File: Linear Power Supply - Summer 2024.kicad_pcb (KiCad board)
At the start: 2 copper layers, 79.5 x 142.5 mm, 4 parts, among them IC1 LD1085V, T1 FP16-3000

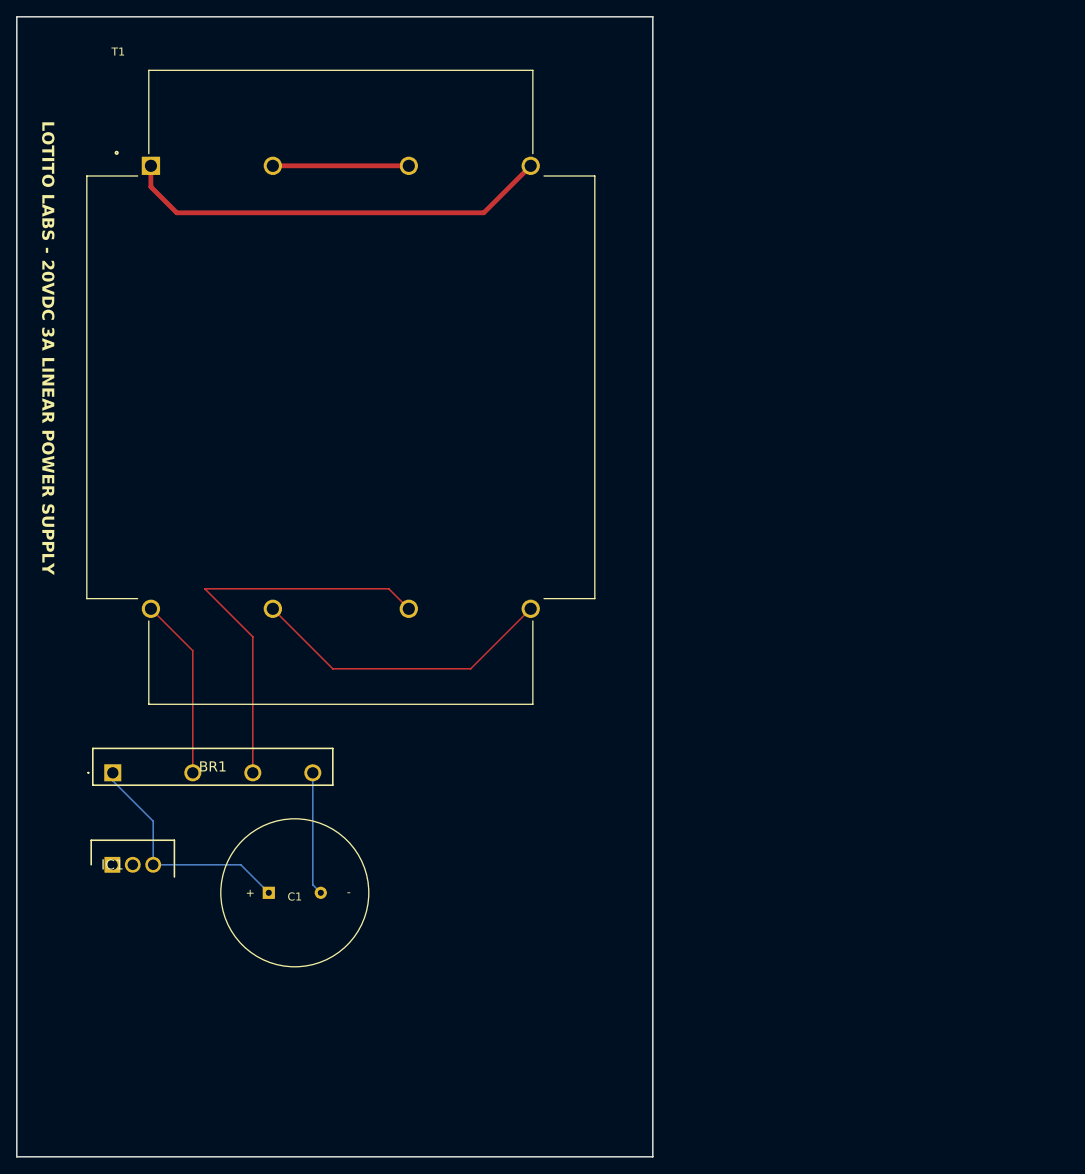
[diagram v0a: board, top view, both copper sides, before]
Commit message: Big push on the PCB layout. I think ready to send to JLC or OSH...
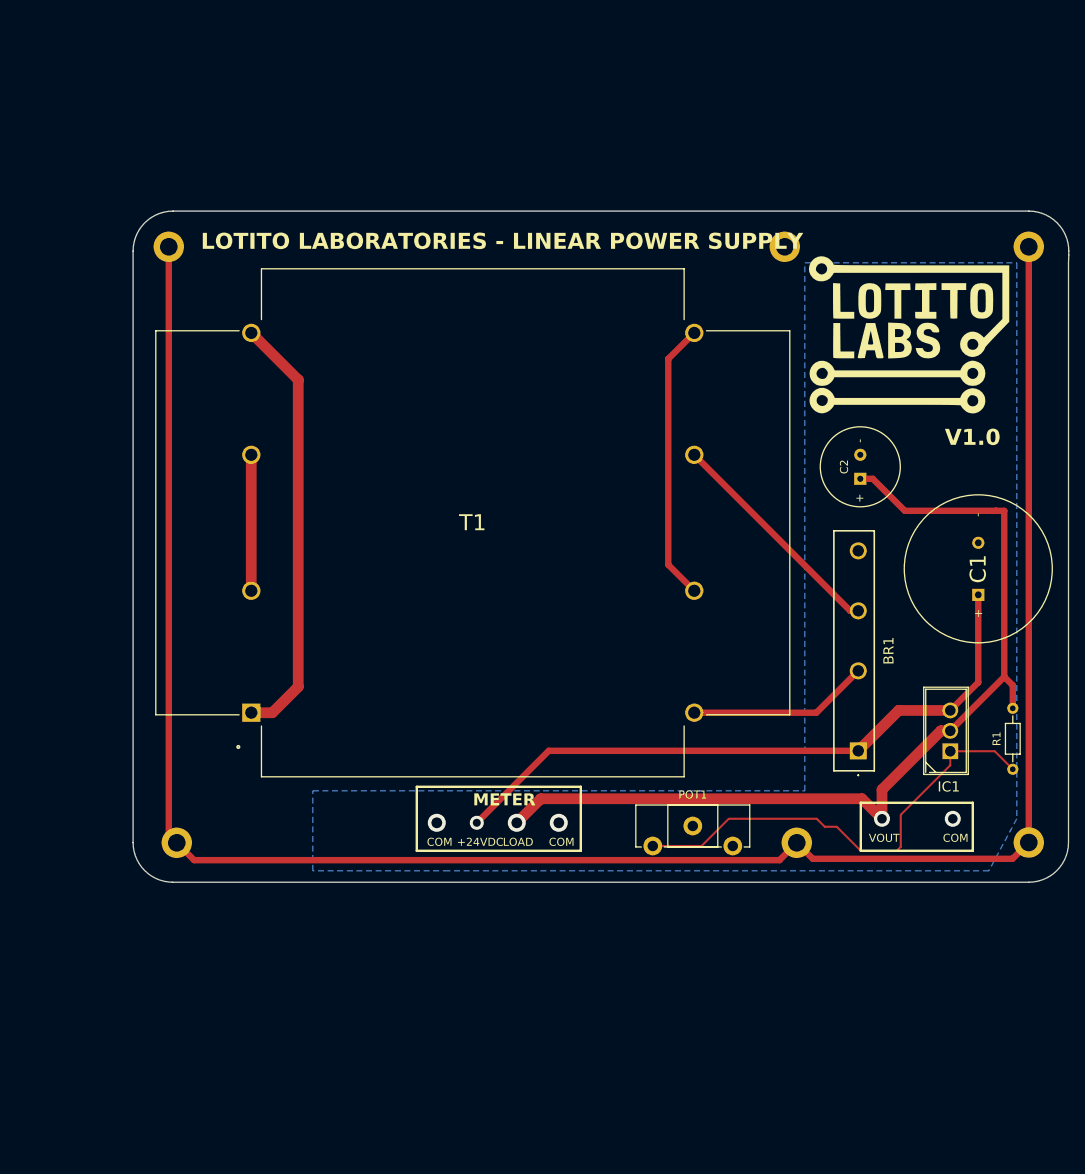
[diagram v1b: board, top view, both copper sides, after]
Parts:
- added C2: 10uF, Chase's Footprints:Small Electrolytic Capacitor, F.Cu at (189.4, 84.5)
- added G***: LOGO, Chase's Footprints:Lotito Labs - 25mm, F.Cu at (195.5, 68.0)
- added POT1: 10k, Potentiometer_THT:Potentiometer_ACP_CA14-H2,5_Horizontal, F.Cu at (163.5, 131.9)
- added R1: 560R, Resistor_THT:R_Axial_DIN0204_L3.6mm_D1.6mm_P7.62mm_Horizontal, F.Cu at (208.5, 114.7)
- added REF**: MountingHole_2.2mm_M2_DIN965_Pad, MountingHole:MountingHole_2.2mm_M2_DIN965_Pad, F.Cu at (104.0, 131.5)
- added REF**: MountingHole_2.2mm_M2_DIN965_Pad, MountingHole:MountingHole_2.2mm_M2_DIN965_Pad, F.Cu at (210.5, 57.0)
- added REF**: MountingHole_2.2mm_M2_DIN965_Pad, MountingHole:MountingHole_2.2mm_M2_DIN965_Pad, F.Cu at (103.0, 57.0)
- added REF**: MountingHole_2.2mm_M2_DIN965_Pad, MountingHole:MountingHole_2.2mm_M2_DIN965_Pad, F.Cu at (181.5, 131.5)
- added REF**: MountingHole_2.2mm_M2_DIN965_Pad, MountingHole:MountingHole_2.2mm_M2_DIN965_Pad, F.Cu at (210.5, 131.5)
- added REF**: MountingHole_2.2mm_M2_DIN965_Pad, MountingHole:MountingHole_2.2mm_M2_DIN965_Pad, F.Cu at (180.0, 57.0)
- moved IC1 105.7 mm to (200.7, 120.1), turned to 90 degrees
- moved C1 94.5 mm to (204.2, 97.3), turned to -90 degrees
- moved BR1 93.2 mm to (189.2, 120.0), turned to 90 degrees
- moved T1 23.6 mm to (141.0, 91.5), turned to 90 degrees
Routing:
- net GND: track 0.00 -> 262.0 mm
- net Vout: track 0.00 -> 117.5 mm, vias 0 -> 2
- net Net-(IC1-ADJ/GND): track 0.00 -> 58.1 mm
- net Net-(BR1-+): track 29.5 -> 81.2 mm, vias 0 -> 1
- net Net-(BR1-~{_2}): track 52.0 -> 28.6 mm
- net COM: track 15.4 -> 0.00 mm, vias 0 -> 3
- net Net-(T1-Pad6): track 38.5 -> 34.9 mm
- added copper zone on B.Cu, net COM
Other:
- board size 79.5 x 142.5 mm -> 117 x 83.9 mm
- board text added: "+24VDC"
- board text added: "COM"
- board text added: "LOAD"
- board text added: "LOTITO LABORATORIES - LINEAR POWER SUPPLY"
- board text added: "METER"
- board text added: "V1.0"
- board text added: "VOUT"
- board text removed: "LOTITO LABS - 20VDC 3A LINEAR POWER SUPPLY"

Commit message: Finished PCB design...
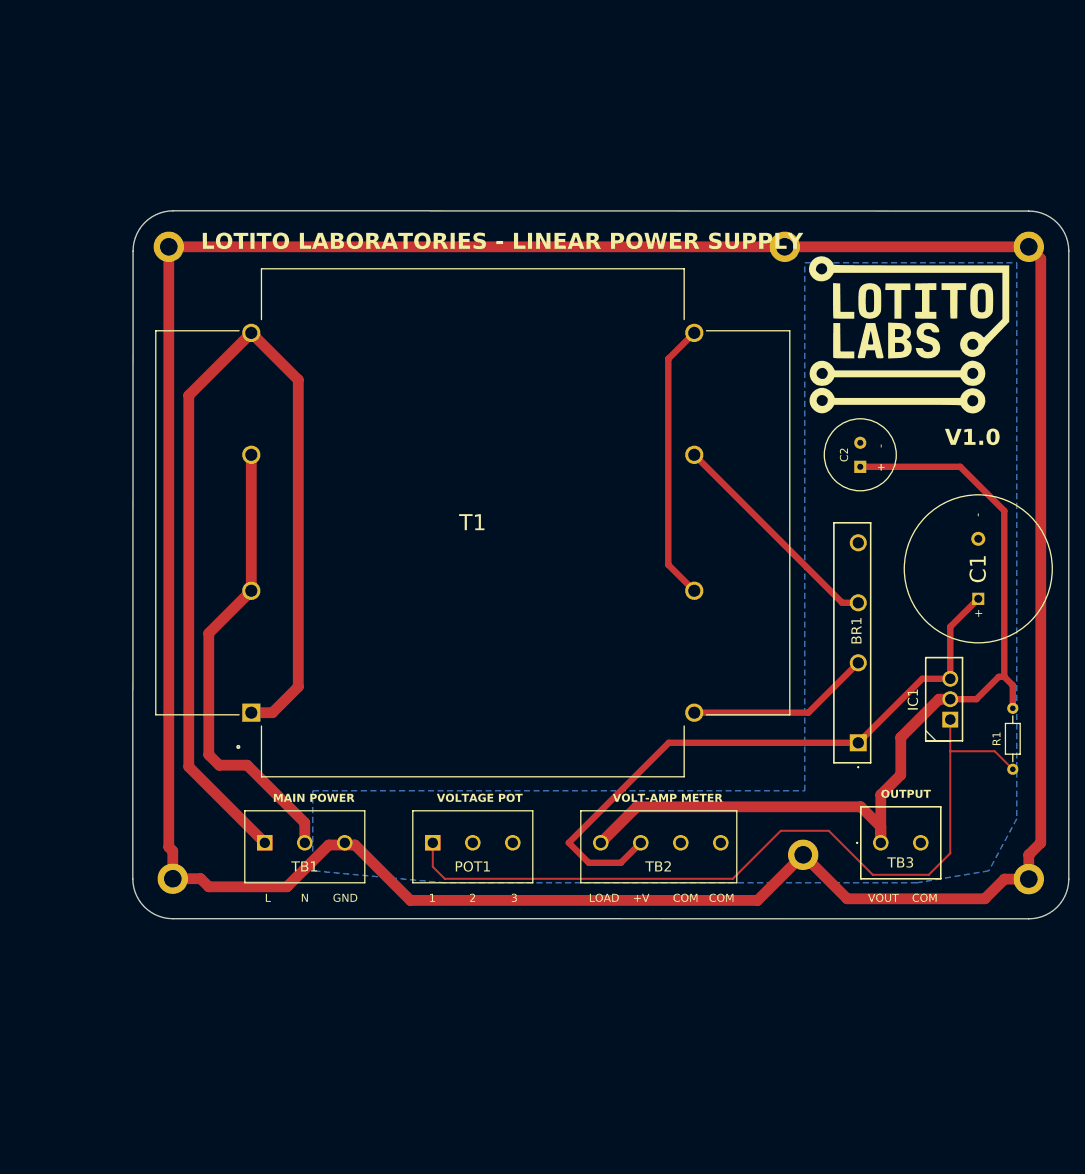
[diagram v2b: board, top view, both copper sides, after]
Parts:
- added TB1: 1935174, SamacSys_PCB_Library:1935174, F.Cu at (115.0, 131.5)
- added TB2: 1935187, SamacSys_PCB_Library:1935187, F.Cu at (157.0, 131.5)
- added TB3: 1935776, SamacSys_PCB_Library:1935776, F.Cu at (192.0, 131.5)
- POT1: footprint Potentiometer_THT:Potentiometer_ACP_CA14-H2,5_Horizontal -> SamacSys_PCB_Library:1935174
- moved POT1 27.5 mm to (136.0, 131.5), turned to 0 degrees
- moved REF** 4.57 mm to (210.5, 136.0)
- moved REF** 4.52 mm to (103.5, 136.0)
- moved IC1 3.95 mm to (200.7, 116.1)
- moved REF** 1.70 mm to (182.3, 133.0)
- moved C2 1.50 mm to (189.4, 83.0)
- moved BR1 1.00 mm to (189.2, 119.0)
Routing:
- net GND: track 262.0 -> 386.5 mm
- net +120VAC/L: track 53.9 -> 124.8 mm
- net Net-(IC1-ADJ/GND): track 58.1 -> 99.6 mm
- net +120VAC/N: track 17.0 -> 57.7 mm
- net Net-(BR1-+): track 81.2 -> 78.7 mm, vias 1 -> 0
- net Vout: track 117.5 -> 115.6 mm, vias 2 -> 0
- net COM: vias 3 -> 0
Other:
- board size 117 x 83.9 mm -> 117 x 88.5 mm
- board text added: "+V"
- board text added: "1"
- board text added: "2"
- board text added: "3"
- board text added: "GND"
- board text added: "L"
- board text added: "MAIN POWER"
- board text added: "N"
- board text added: "OUTPUT"
- board text added: "VOLT-AMP METER"
- board text added: "VOLTAGE POT"
- board text removed: "+24VDC"
- board text removed: "METER"
